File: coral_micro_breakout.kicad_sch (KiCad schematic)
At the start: 3 parts, among them J1 Conn_01x03_Socket

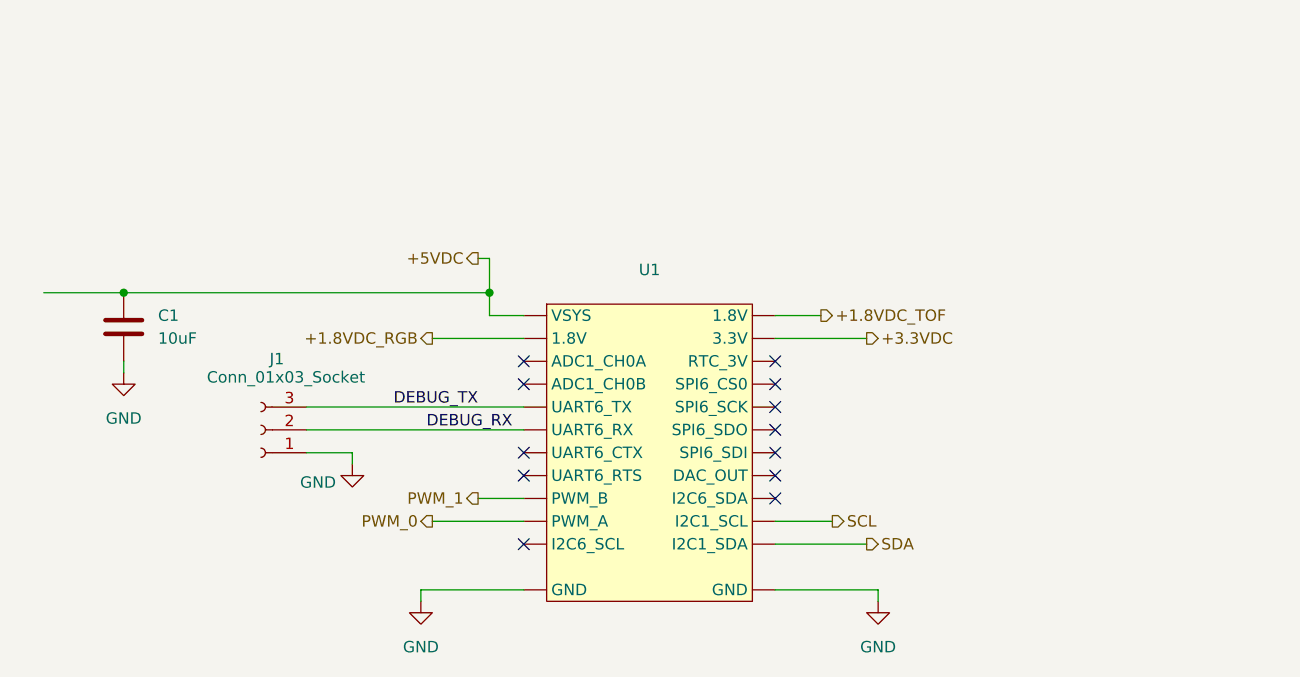
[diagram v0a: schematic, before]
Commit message: working on board
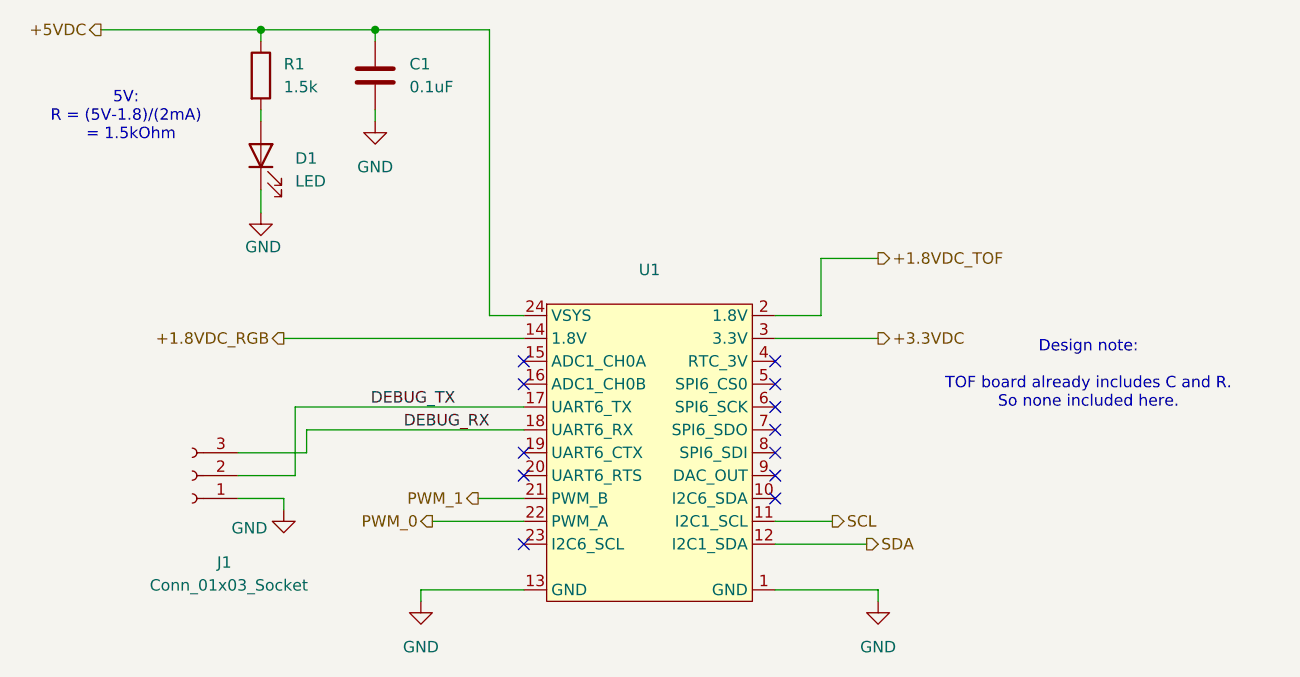
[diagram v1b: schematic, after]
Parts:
- added D1: LED, LED_SMD:LED_0805_2012Metric_Pad1.15x1.40mm_HandSolder, symbol Device:LED
- added R1: 1.5k, Resistor_SMD:R_0805_2012Metric_Pad1.20x1.40mm_HandSolder, symbol Device:R
- C1: value 10uF -> 0.1uF; footprint (none) -> Capacitor_SMD:C_0504_1310Metric_Pad0.83x1.28mm_HandSolder
- J1: footprint (none) -> Connector_PinHeader_2.54mm:PinHeader_1x03_P2.54mm_Vertical
- U1: footprint (none) -> 00_parts_lib:coral_micro_board_mating
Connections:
- net +1.8VDC_RGB: now also U1.14 (1.8V); no longer U1. (VSYS)
- net +1.8VDC_TOF: now also U1.2 (1.8V); no longer U1. (VSYS)
- net +3.3VDC: now also U1.3 (3.3V); no longer U1. (VSYS)
- net +5VDC: now also C1.2, U1.24 (VSYS), R1.1; no longer C1.1, U1. (VSYS)
- net DEBUG_RX: now also J1.3 (Pin_3), U1.18 (UART6_RX); no longer J1.2 (Pin_2), U1. (VSYS)
- net DEBUG_TX: now also J1.2 (Pin_2), U1.17 (UART6_TX); no longer J1.3 (Pin_3), U1. (VSYS)
- net GND: now also C1.1, U1.1 (GND), U1.13 (GND), D1.1 (K); no longer C1.2, U1. (VSYS)
- net PWM_0: now also U1.22 (PWM_A); no longer U1. (VSYS)
- net PWM_1: now also U1.21 (PWM_B); no longer U1. (VSYS)
- net SCL: now also U1.11 (I2C1_SCL); no longer U1. (VSYS)
- net SDA: now also U1.12 (I2C1_SDA); no longer U1. (VSYS)
- new net: D1.2 (A), R1.2
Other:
- note added: "5V: R = (5V-1.8)/(2mA) = 1.5kOhm"
- note added: "Design note: TOF board already includes C and R. So none included here."
- moved on the sheet: J1
